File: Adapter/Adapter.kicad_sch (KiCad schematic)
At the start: 11 parts, among them J2 Conn_01x14_Socket, U1 BGA153 UFS Adapter Modified

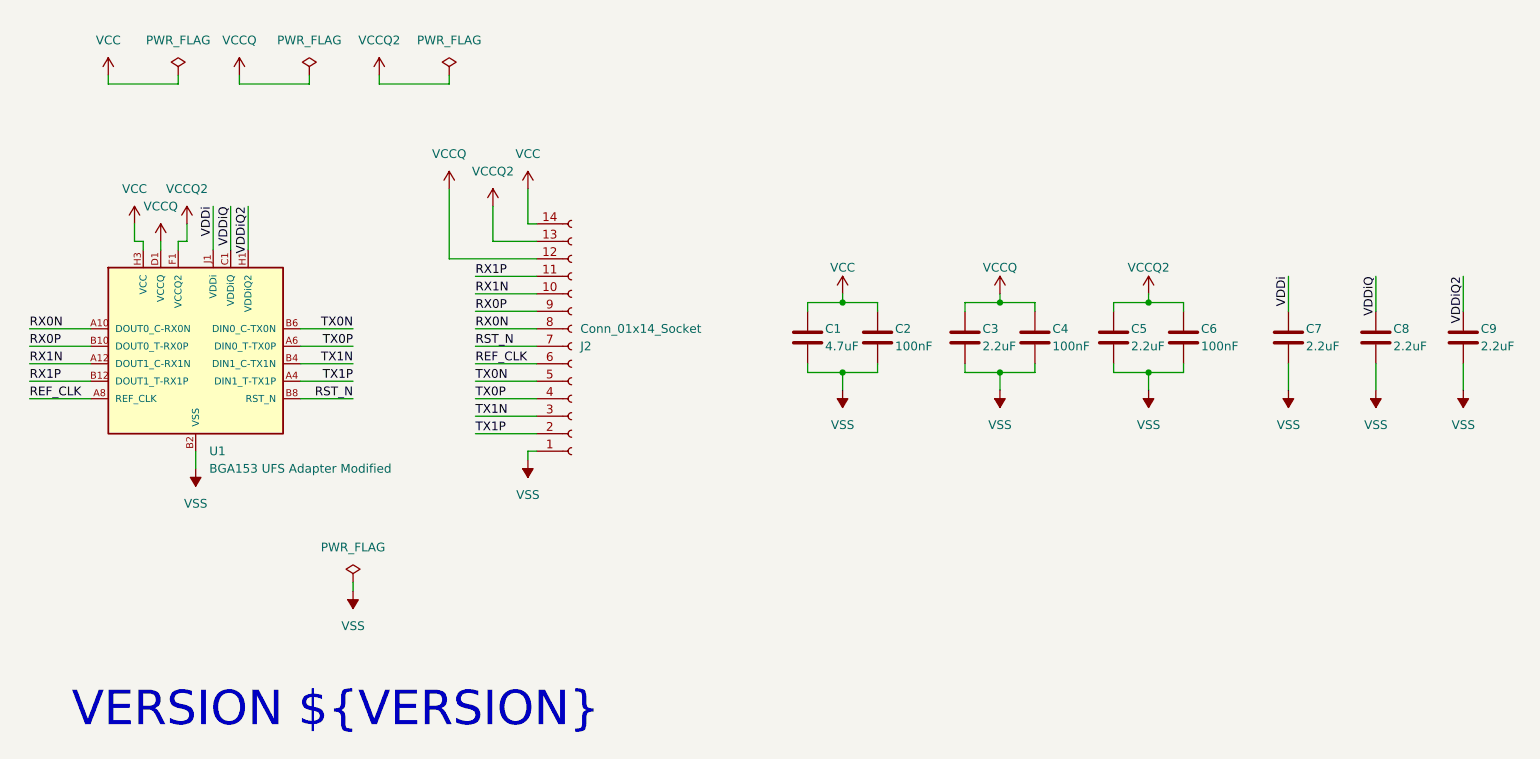
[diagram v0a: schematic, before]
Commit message: V1.3 GB042 Connector
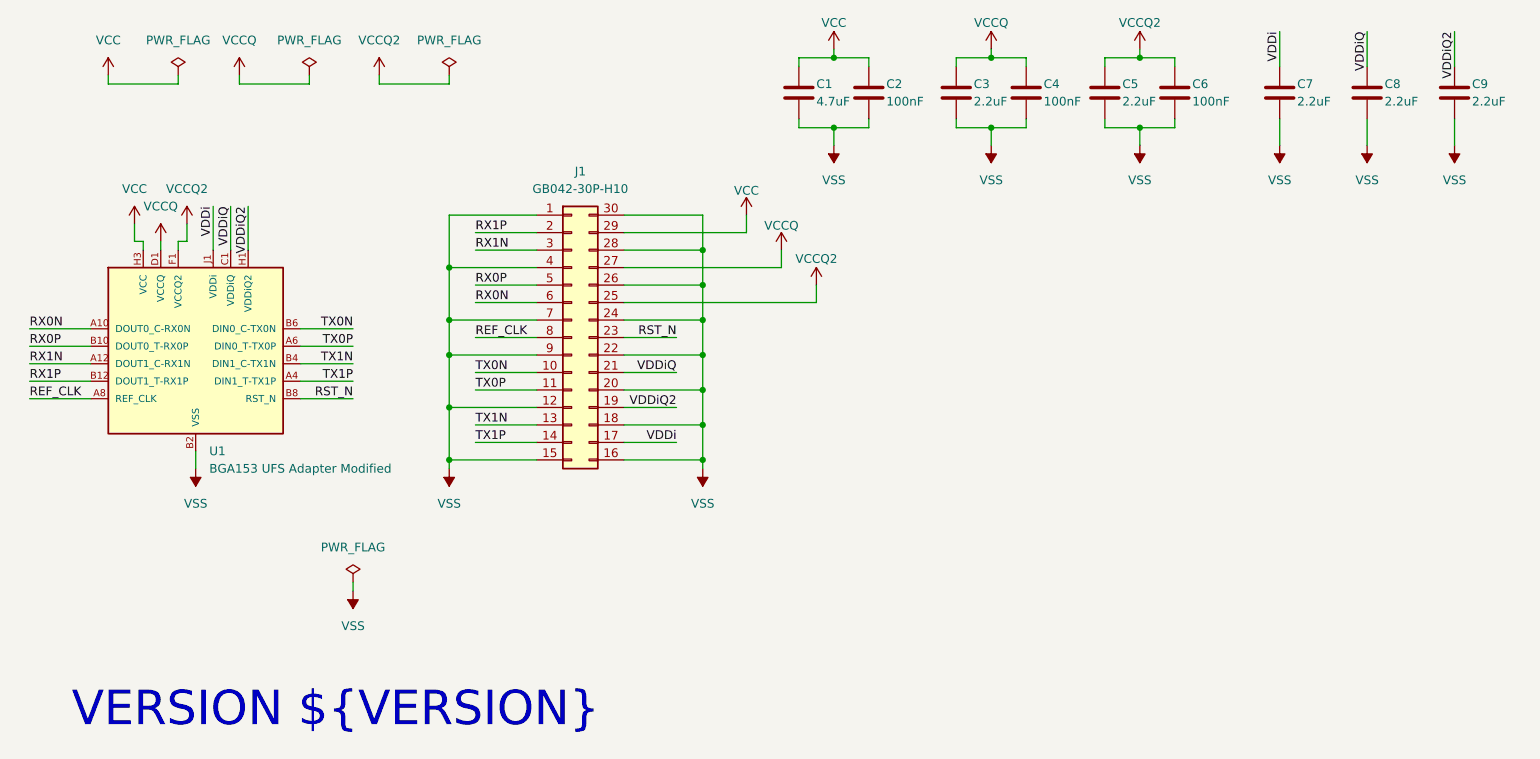
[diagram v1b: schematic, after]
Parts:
- removed J2: Conn_01x14_Socket, BGA153:FPC 14 Pin 0.5P, symbol Connector:Conn_01x14_Socket
- added J1: GB042-30P-H10, BGA153:GB042-30P-H10, symbol BGA153:GB042-30P-H10
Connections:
- net REF_CLK: now also J1.8 (Pin_8)
- net RST_N: now also J1.23 (Pin_23)
- net RX0N: now also J1.6 (Pin_6)
- net RX0P: now also J1.5 (Pin_5)
- net RX1N: now also J1.3 (Pin_3)
- net RX1P: now also J1.2 (Pin_2)
- net TX0N: now also J1.10 (Pin_10)
- net TX0P: now also J1.11 (Pin_11)
- net TX1N: now also J1.13 (Pin_13)
- net TX1P: now also J1.14 (Pin_14)
- net VCC: now also J1.29 (Pin_29)
- net VCCQ: now also J1.27 (Pin_27)
- net VCCQ2: now also J1.25 (Pin_25)
- net VDDi: now also J1.17 (Pin_17)
- net VDDiQ: now also J1.21 (Pin_21)
- net VDDiQ2: now also J1.19 (Pin_19)
- net VSS: now also J1.1 (Pin_1), J1.12 (Pin_12), J1.15 (Pin_15), J1.16 (Pin_16), J1.18 (Pin_18), J1.20 (Pin_20), J1.22 (Pin_22), J1.24 (Pin_24), J1.26 (Pin_26), J1.28 (Pin_28), J1.30 (Pin_30), J1.4 (Pin_4), J1.7 (Pin_7), J1.9 (Pin_9)
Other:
- moved on the sheet: C1, C2, C3, C4, C5, C6, C7, C8, C9
